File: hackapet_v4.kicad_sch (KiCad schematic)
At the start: 43 parts, among them J1 Conn_01x02_Socket, J4 USB_C_Receptacle_USB2.0_16P, J7 lipo, Q1 AO3401A, SW1 SW_Push, SW2 SW_Push, SW3 SW_Push, SW4 SW_SPDT, U1 XC6206PxxxMR, U2 ESP-PSRAM32, U3 ESP32-S2-MINI-2, U9 TP4056-42-ESOP8

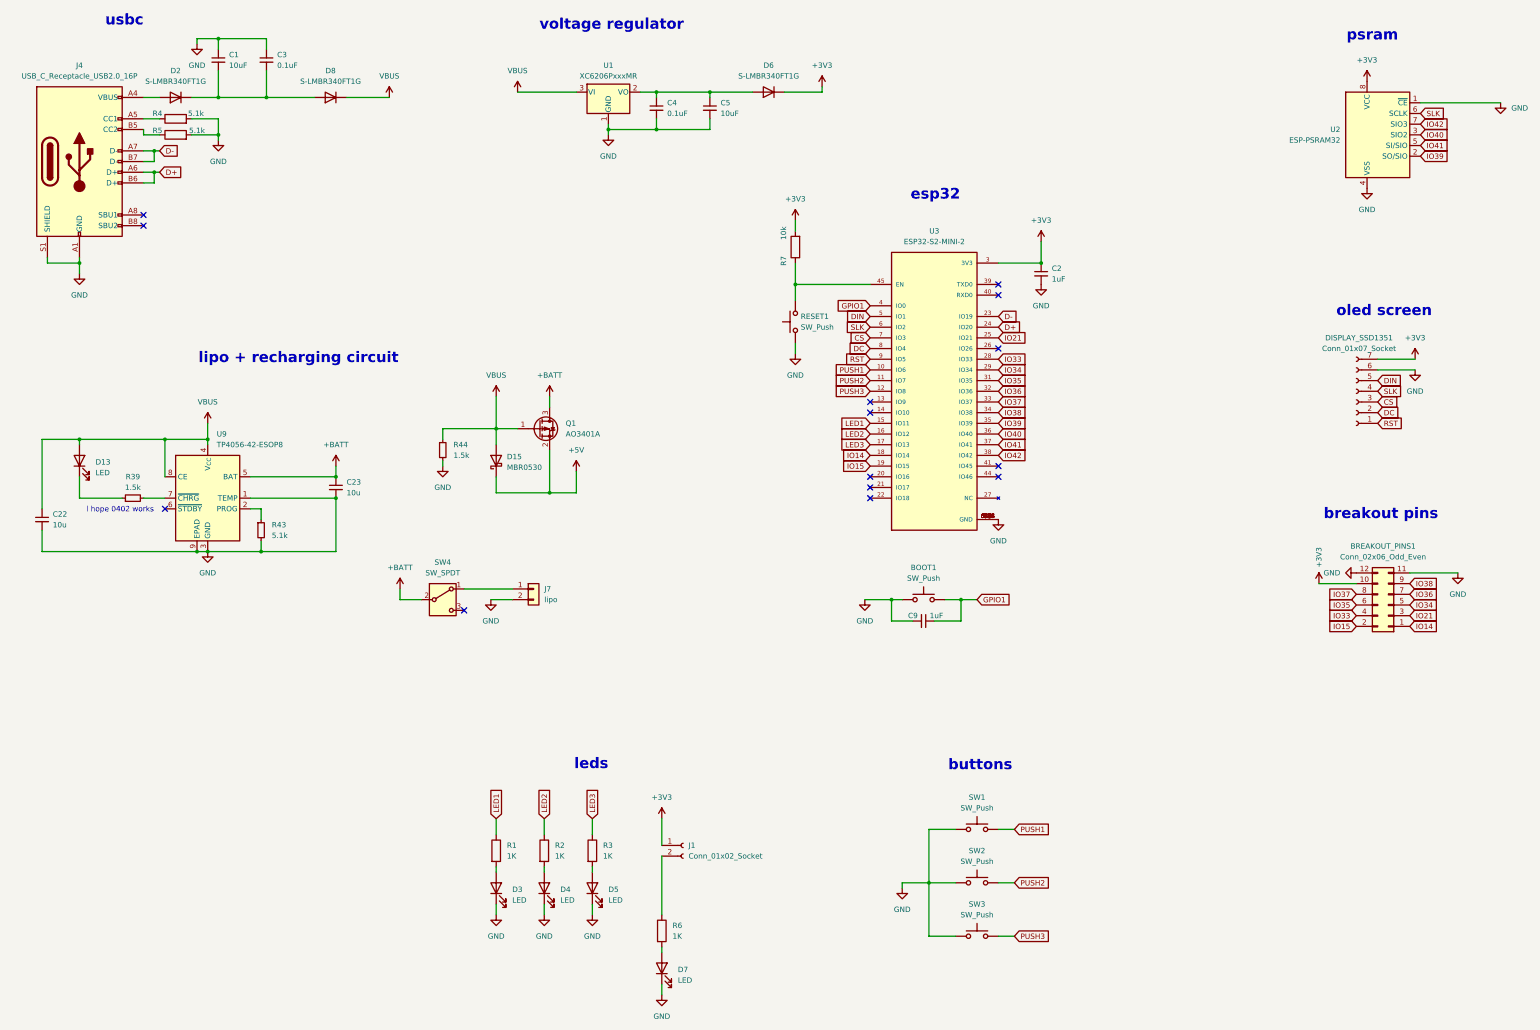
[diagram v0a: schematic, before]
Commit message: routed!
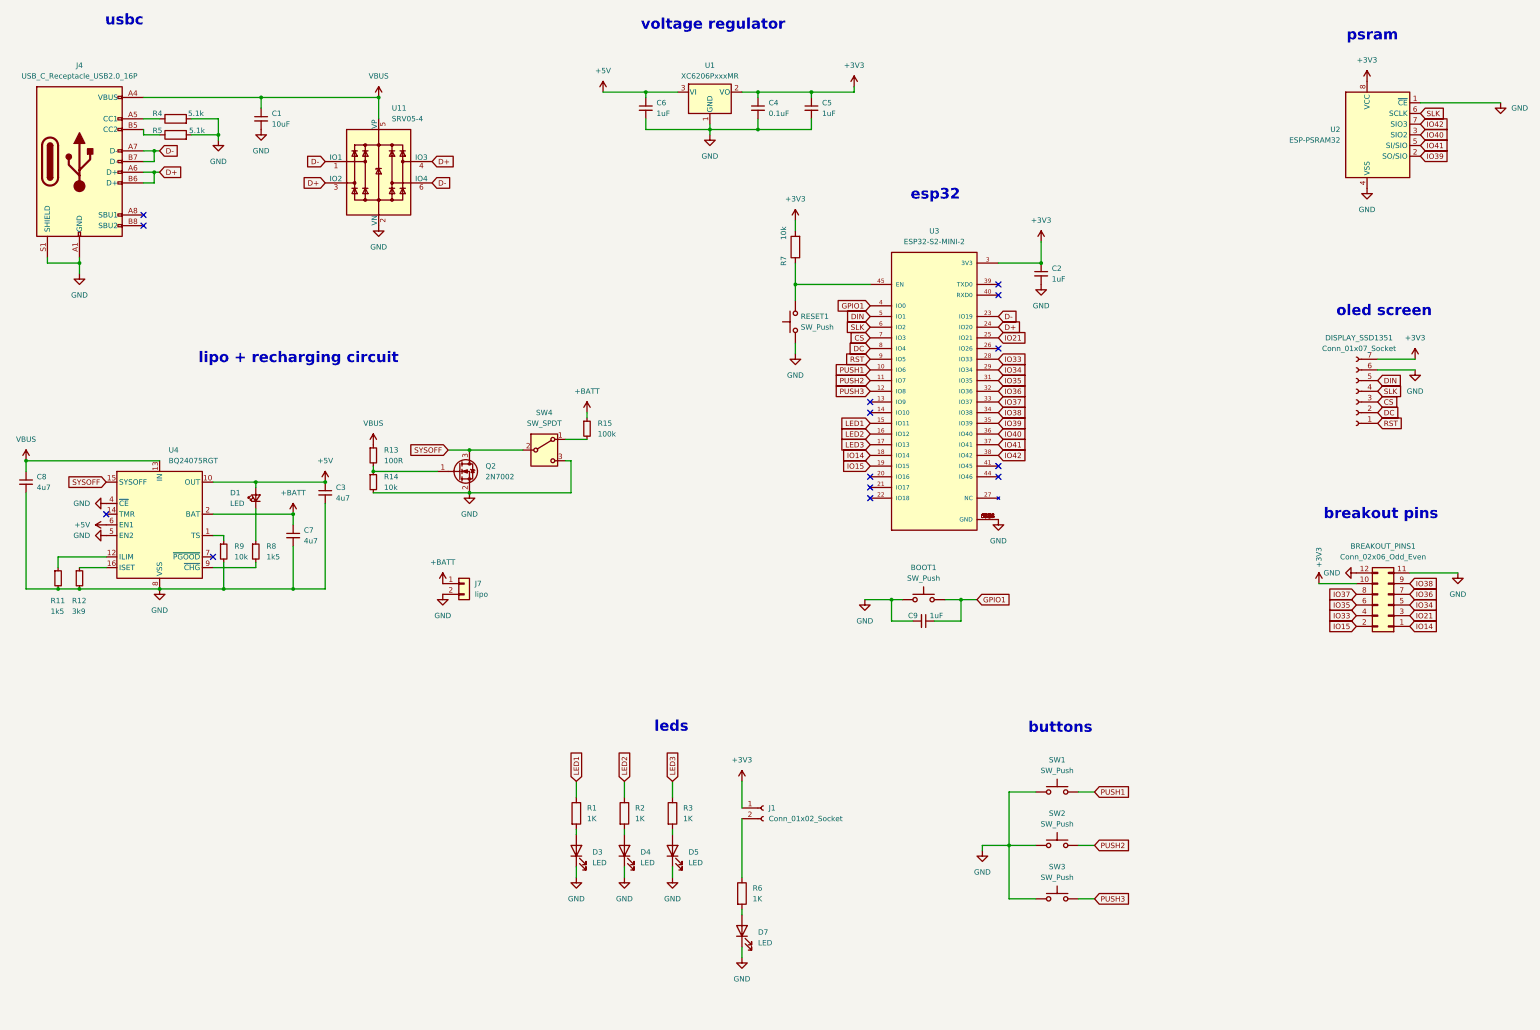
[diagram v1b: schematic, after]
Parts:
- removed C22, C23: 10u, Capacitor_SMD:C_0805_2012Metric, symbol Device:C_Small
- removed D13: LED, LED_SMD:LED_0805_2012Metric, symbol Device:LED
- removed D15: MBR0530, Diode_SMD:D_SOD-123, symbol Diode:MBR0530
- removed D2, D6, D8: S-LMBR340FT1G, Diode_SMD:D_0805_2012Metric, symbol Device:D
- removed Q1: AO3401A, Package_TO_SOT_SMD:SOT-23, symbol Transistor_FET:AO3401A
- removed R39, R44: 1.5k, Resistor_SMD:R_0805_2012Metric, symbol Device:R_Small
- removed R43: 5.1k, Resistor_SMD:R_0805_2012Metric, symbol Device:R_Small
- removed U9: TP4056-42-ESOP8, Package_SO:SOIC-8-1EP_3.9x4.9mm_P1.27mm_EP2.41x3.3mm_ThermalVias, symbol Battery_Management:TP4056-42-ESOP8
- added C6: 1uF, Capacitor_SMD:C_0805_2012Metric, symbol Device:C_Small
- added C7, C8: 4u7, Capacitor_SMD:C_0805_2012Metric, symbol Device:C_Small
- added D1: LED, LED_SMD:LED_0805_2012Metric, symbol Device:LED_Small
- added Q2: 2N7002, Package_TO_SOT_SMD:SOT-23, symbol Transistor_FET:2N7002
- added R11, R8: 1k5, Resistor_SMD:R_0805_2012Metric, symbol Device:R_Small
- added R12: 3k9, Resistor_SMD:R_0805_2012Metric, symbol Device:R_Small
- added R13: 100R, Resistor_SMD:R_0805_2012Metric, symbol Device:R_Small
- added R14, R9: 10k, Resistor_SMD:R_0805_2012Metric, symbol Device:R_Small
- added R15: 100k, Resistor_SMD:R_0805_2012Metric, symbol Device:R_Small
- added U11: SRV05-4, Package_TO_SOT_SMD:SOT-23-6, symbol Power_Protection:SRV05-4
- added U4: BQ24075RGT, Package_DFN_QFN:VQFN-16-1EP_3x3mm_P0.5mm_EP1.6x1.6mm, symbol Battery_Management:BQ24075RGT
- C3: value 0.1uF -> 4u7; LCSC C28378 -> (none)
- C5: value 10uF -> 1uF
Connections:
- net +3V3: now also C4.1, C5.1, U1.2 (VO)
- net +5V: now also C3.1, U1.3 (VI), C6.1, D1.2 (A), U4.10 (OUT), U4.11 (OUT), U4.6 (EN1)
- net +BATT: now also J7.1 (Pin_1), C7.1, R15.1, U4.2 (BAT), U4.3 (BAT); no longer SW4.2 (B)
- net D+: now also U11.3 (IO2), U11.4 (IO3)
- net D-: now also U11.1 (IO1), U11.6 (IO4)
- net GND: now also C1.2, C3.2, SW4.3 (C), C6.2, C7.2, C8.2, Q2.2 (S), R11.2, R12.2, R14.2, R9.2, U11.2 (VN), U4.17 (VSS), U4.4 (~{CE}), U4.5 (EN2), U4.8 (VSS); no longer C1.1, C3.1
- net VBUS: now also C1.1, J4.A4 (VBUS), J4.A9 (VBUS), J4.B4 (VBUS), J4.B9 (VBUS), C8.1, R13.1, U11.5 (VP), U4.13 (IN); no longer U1.3 (VI)
- net at SW4.1 (A): now also R15.2; no longer J7.1 (Pin_1)
- new net: Q2.1 (G), R13.2, R14.1
- new net: D1.1 (K), R8.1
- new net: R8.2, U4.9 (~{CHG})
- new net: R11.1, U4.12 (ILIM)
- new net: R9.1, U4.1 (TS)
- new net: R12.1, U4.16 (ISET)
- new net SYSOFF: Q2.3 (D), SW4.2 (B), U4.15 (SYSOFF)
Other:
- note removed: "i hope 0402 works"
- moved on the sheet: C1, C4, C5, D3, D4, D5, D7, J1, J7, R1, R2, R3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
